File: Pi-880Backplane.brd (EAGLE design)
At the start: 105.4 x 71.1 mm, 2 parts

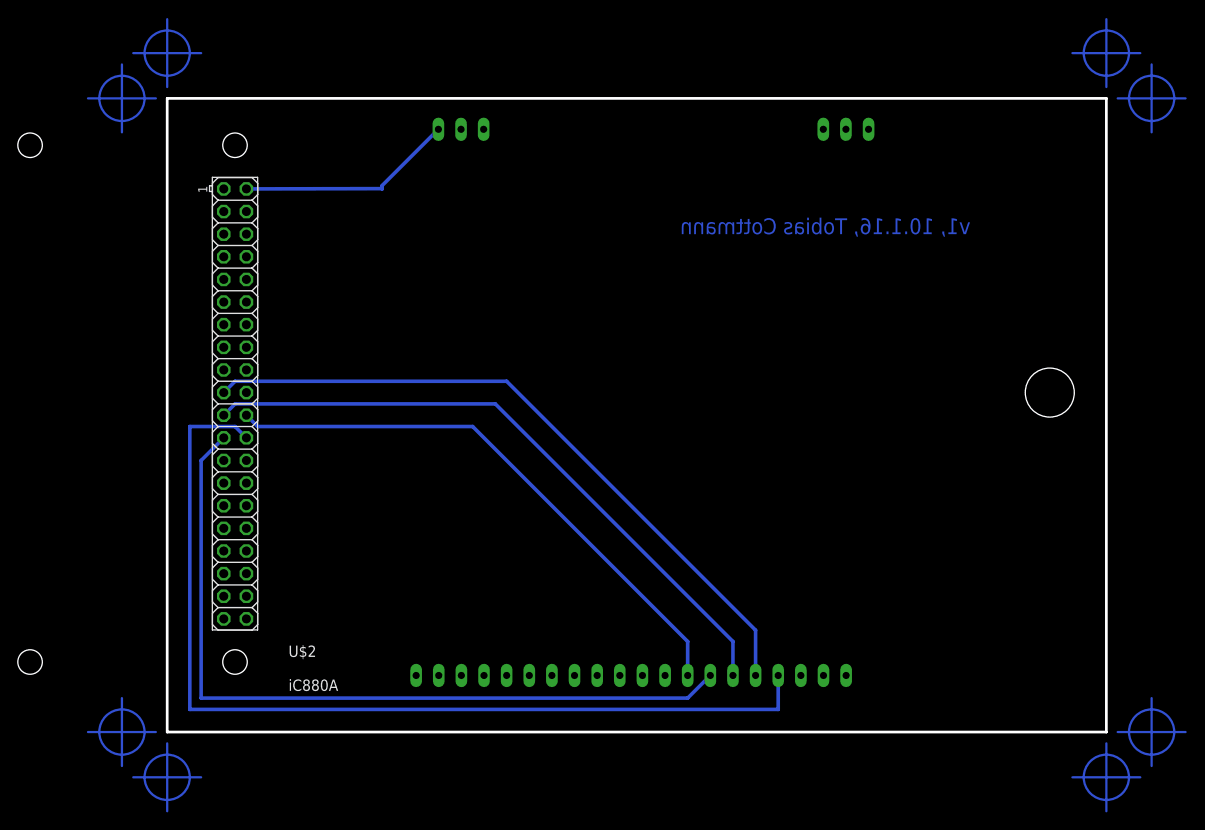
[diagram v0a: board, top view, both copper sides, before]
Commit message: Merged v2
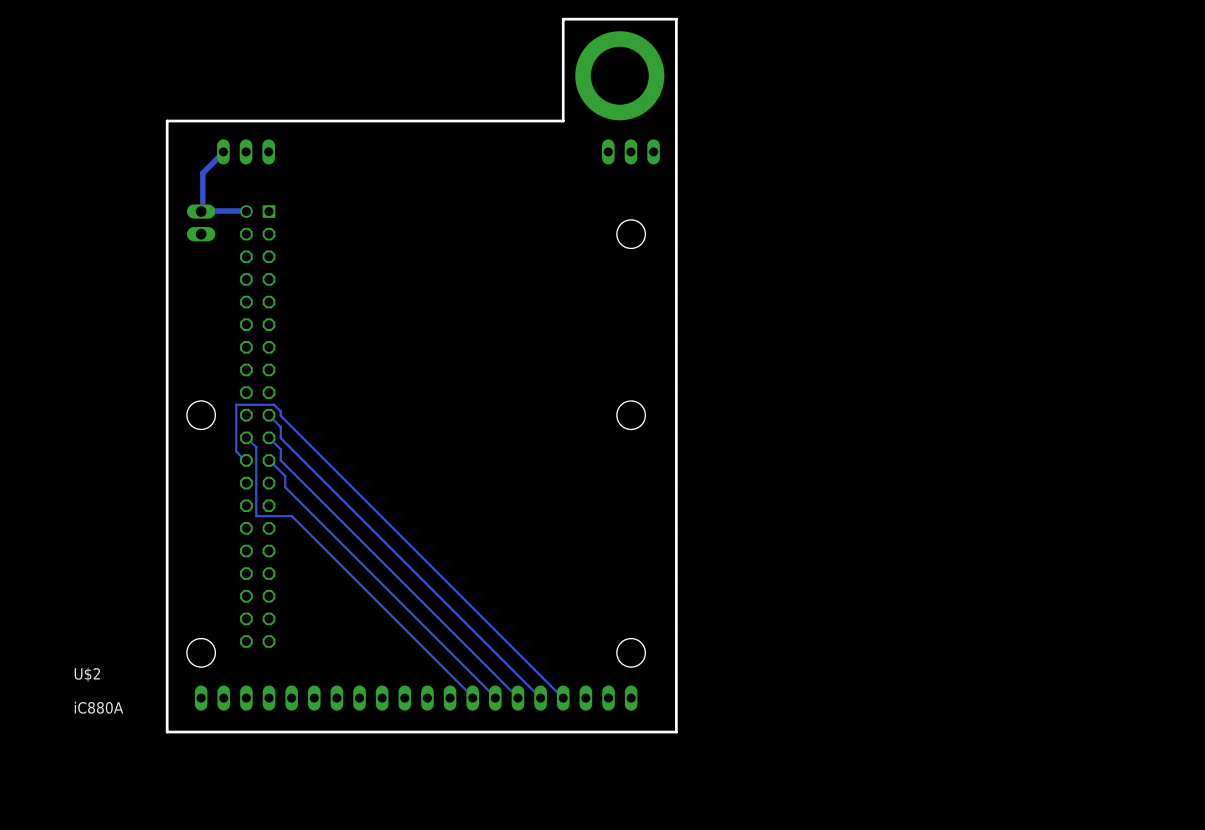
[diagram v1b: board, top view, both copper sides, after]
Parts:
- added U$3: SMA-PIGTAIL-MOUNT, tobias:SMA-PIGTAIL-MOUNT
- added X1: (no value), con-phoenix-254:2POL254
- U$1: value RPI-ZERO -> RPI-ZERONODRILLS; device RPI-Zero:RASPBERRYPI_BASTELSTUBE_V13_RASPI_BOARD_B+_FULL -> tobias:RPI-ZERO-NODRILLS
- moved U$1 55.9 mm to (36.8, 67.3), flipped to the bottom
- moved U$2 24.3 mm to (-12.7, 0.00)
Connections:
- net GND: now also U$3.GND, X1.2
- net VCC: now also X1.1
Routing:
- net SPI_CLK: track 88.5 -> 37.2 mm
- net NSS: track 108.5 -> 57.4 mm
- net MOSI: track 76.9 -> 44.4 mm
- net MISO: track 72.5 -> 40.8 mm
- net RESET: track 63.9 -> 42.1 mm
- net VCC: track 24.6 -> 12.7 mm
- net N$6: track 7.62 -> 0.00 mm
- net N$2: track 7.62 -> 0.00 mm
- net N$16: track 7.62 -> 0.00 mm
- net N$13: track 7.62 -> 0.00 mm
- net N$12: track 7.62 -> 0.00 mm
- net N$11: track 7.62 -> 0.00 mm
- net N$3: track 7.62 -> 0.00 mm
- net N$14: track 7.62 -> 0.00 mm
- net N$10: track 7.62 -> 0.00 mm
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- added copper zone on layer 1, net GND
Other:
- board size 105.4 x 71.1 mm -> 57.1 x 80 mm
- board text removed: "v1, 10.1.16, Tobias Cottmann"
